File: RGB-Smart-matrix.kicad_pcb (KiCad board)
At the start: 2 copper layers, 41.1 x 43 mm, 187 parts, among them J2 Conn_01x07_Pin, J3 Conn_01x06_Pin

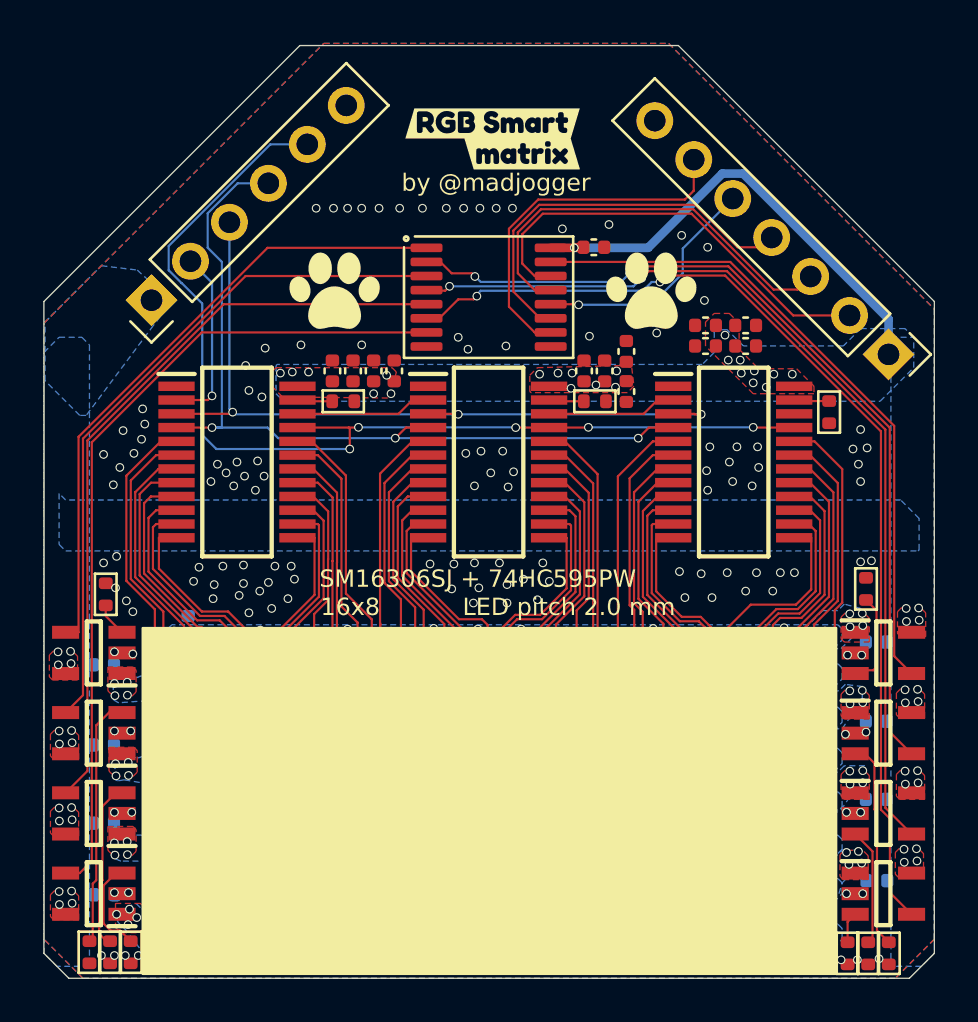
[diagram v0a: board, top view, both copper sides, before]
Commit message: drc fix
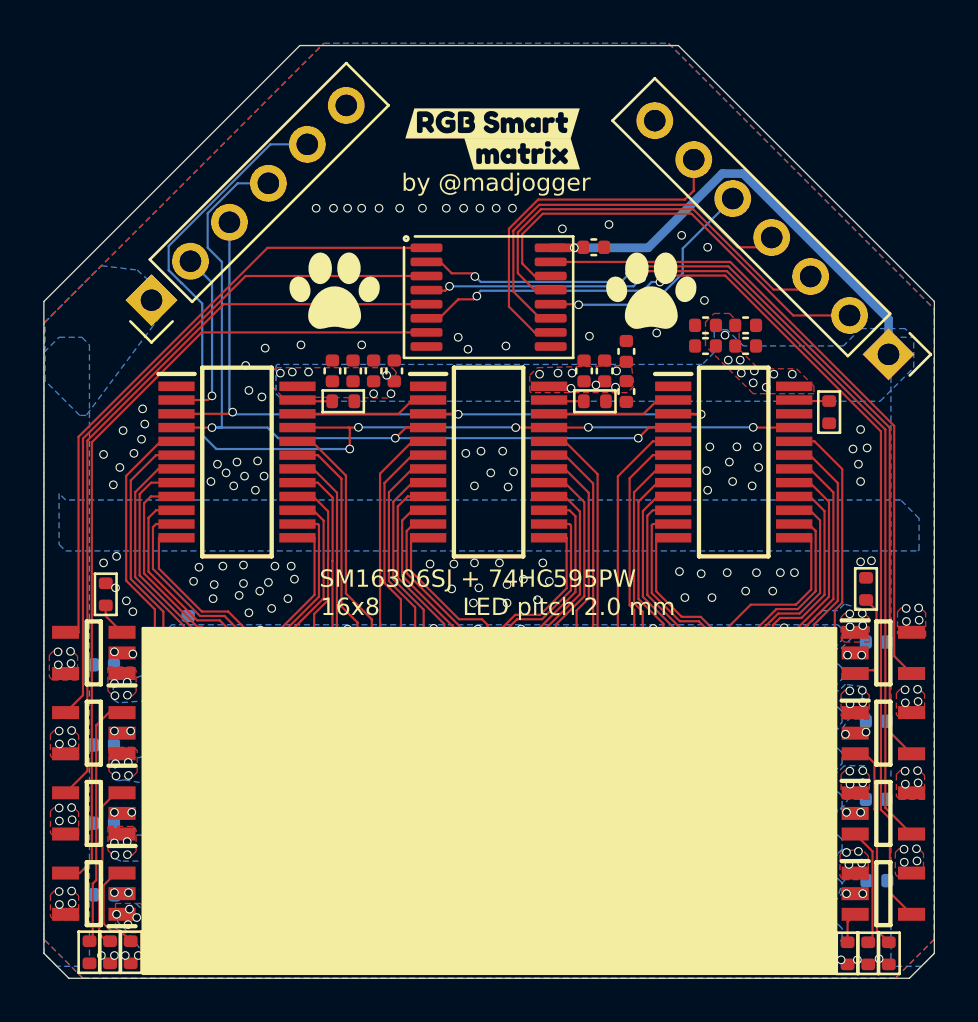
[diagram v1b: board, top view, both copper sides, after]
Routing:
- net BLUE8: track 26.5 -> 24.4 mm
